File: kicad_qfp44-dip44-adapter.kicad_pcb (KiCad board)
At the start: 2 copper layers, 57.4 x 21.8 mm, 4 parts, among them J1 Conn_01x22_Male, J2 Conn_01x22_Male, U1 QFP44

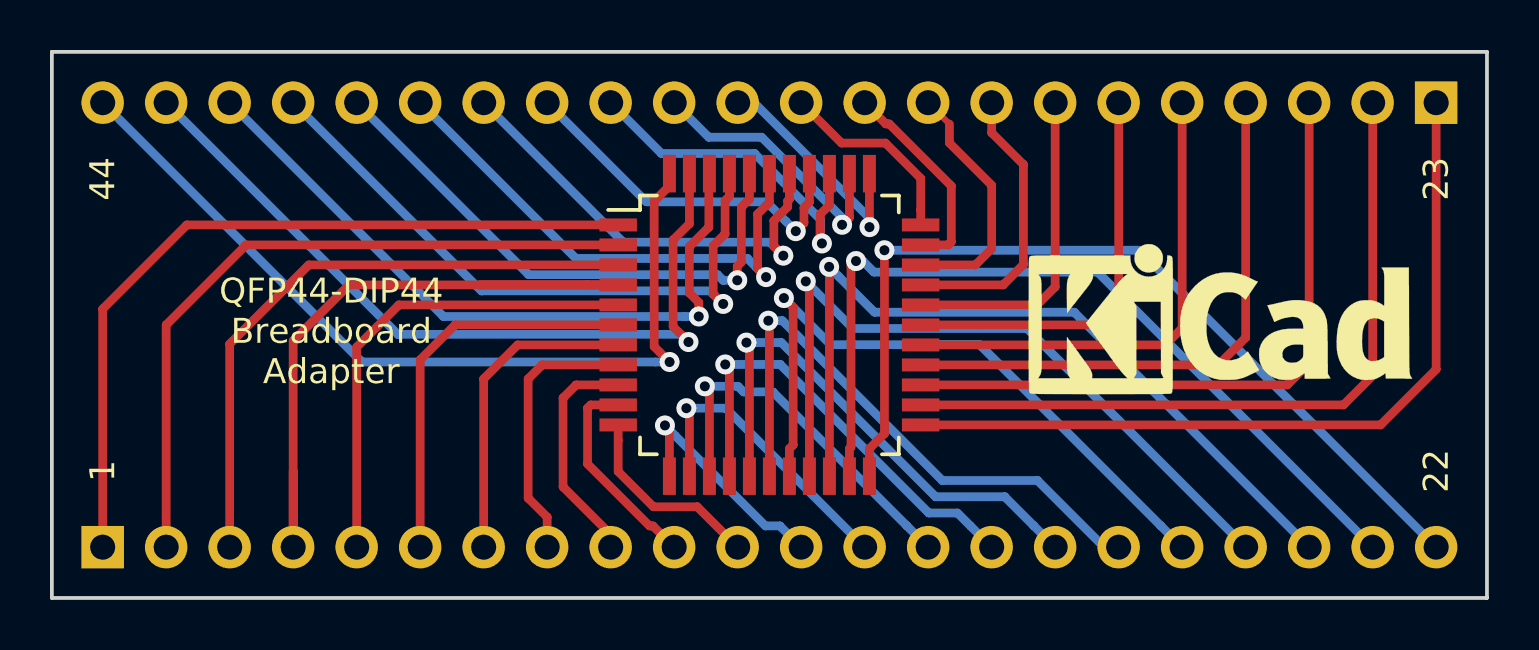
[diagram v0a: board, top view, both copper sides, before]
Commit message: Beautification
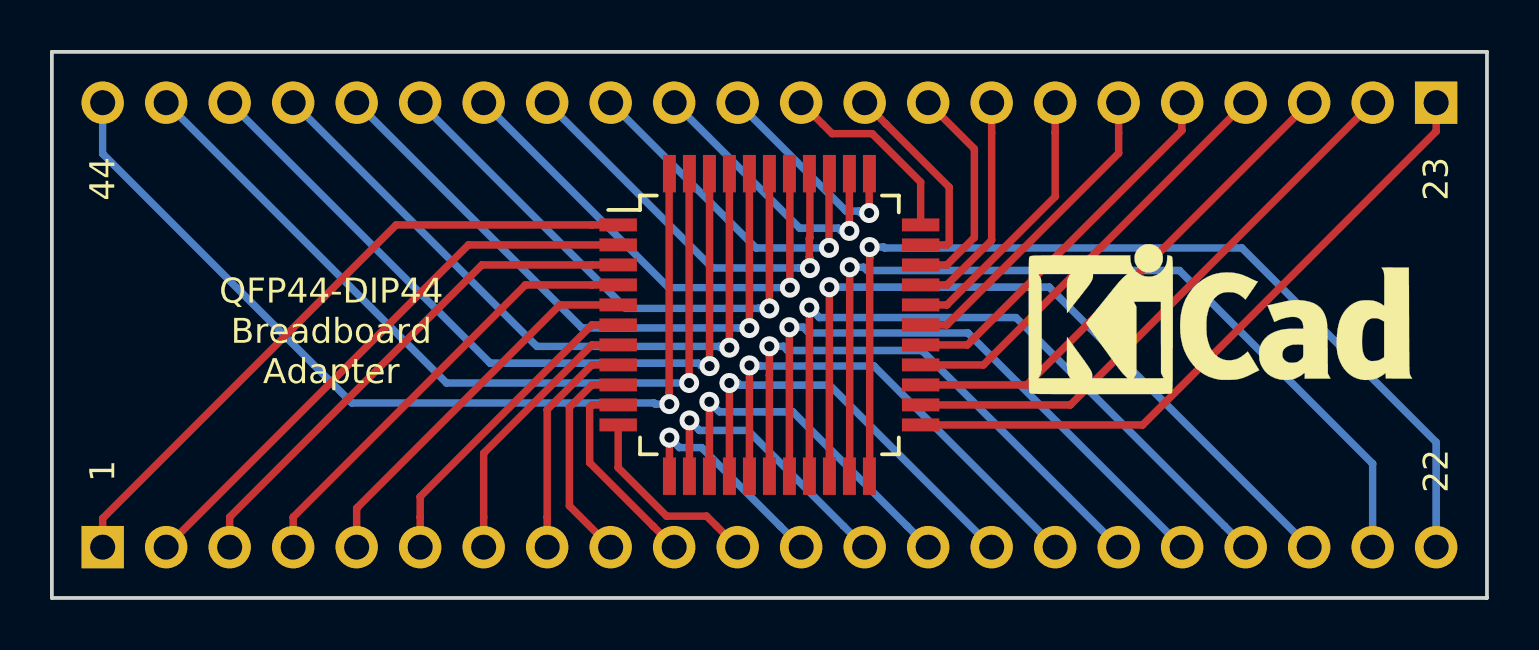
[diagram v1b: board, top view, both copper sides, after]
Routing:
- net 4: track 32.1 -> 18.0 mm
- net 24: track 29.5 -> 23.1 mm
- net 25: track 26.3 -> 20.2 mm
- net 23: track 32.2 -> 26.6 mm
- net 26: track 22.9 -> 17.3 mm
- net 2: track 28.3 -> 23.1 mm
- net 1: track 31.5 -> 26.6 mm
- net 27: track 19.8 -> 15.1 mm
- net 3: track 25.0 -> 20.9 mm
- net 28: track 16.6 -> 12.8 mm
- net 5: track 19.2 -> 15.4 mm
- net 6: track 16.0 -> 12.8 mm
- net 44: track 35.0 -> 38.1 mm
- net 40: track 22.6 -> 25.6 mm
- net 22: track 36.3 -> 39.3 mm
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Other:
- net class Default: clearance 0.3 -> 0.24; trace_width 0.35 -> 0.3
- rule trace_clearance: 0.3 -> 0.24
